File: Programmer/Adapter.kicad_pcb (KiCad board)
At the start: 2 copper layers, 38.1 x 20.3 mm, 5 parts, among them IC1 ARDUINO_PRO_MINI_BASIC, P1 CONN_01X06, P2 CONN_01X02, SW1 SWITCH_SPDT, SW2 SWITCH_SPDT

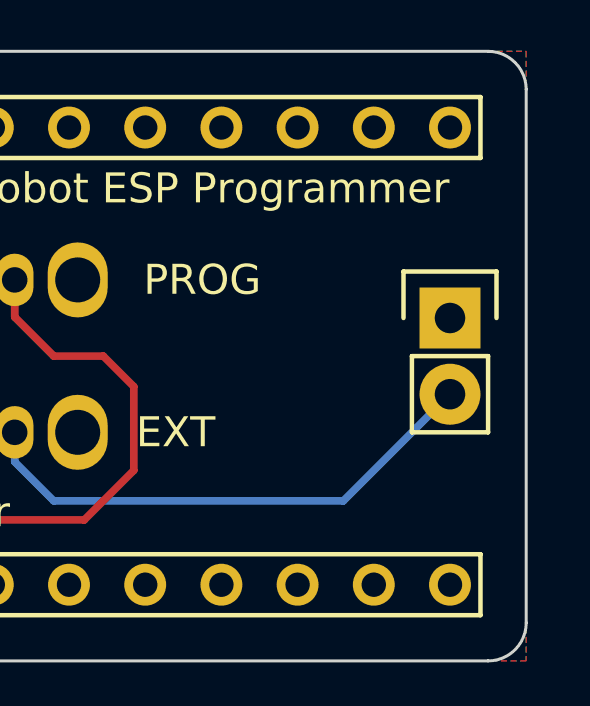
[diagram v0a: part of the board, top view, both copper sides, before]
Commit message: Final production release for v2
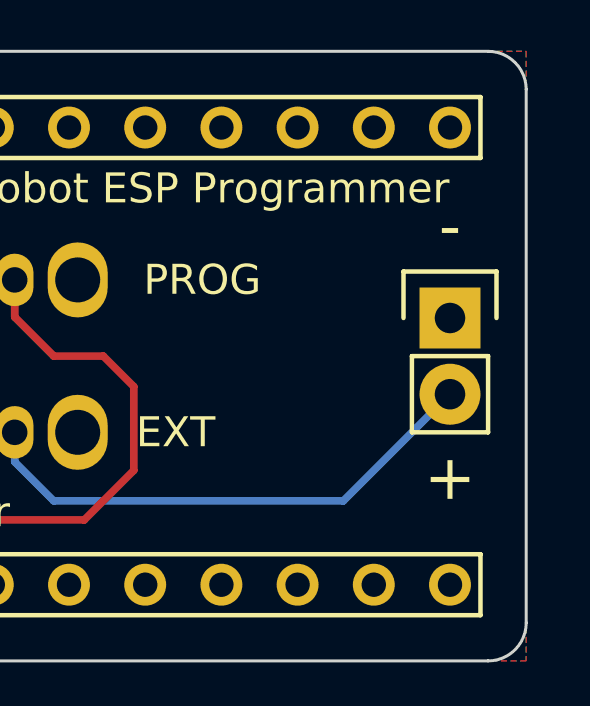
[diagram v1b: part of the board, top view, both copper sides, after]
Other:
- board text added: "+"
- board text added: "-"
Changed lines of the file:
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@@
     (links 10)
     (no_connects 0)
-    (area 128.219999 93.929999 166.420001 114.350001)
+    (area 125.647667 91.511 168.992334 114.350001)
     (thickness 1.6)
-    (drawings 20)
+    (drawings 24)
     (tracks 28)
     (zones 0)
@@
     (pad 5 thru_hole oval (at -4.1 0) (size 2 2.5) (drill 1.5) (layers *.Cu *.Mask F.SilkS))
   )
+  (dimension 20.32 (width 0.3) (layer Eco1.User)
+    (gr_text "20.320 mm" (at 170.768 104.14 270) (layer Eco1.User)
+      (effects (font (size 1.5 1.5) (thickness 0.3)))
+    )
+    (feature1 (pts (xy 167.132 114.3) (xy 172.118 114.3)))
+    (feature2 (pts (xy 167.132 93.98) (xy 172.118 93.98)))
+    (crossbar (pts (xy 169.418 93.98) (xy 169.418 114.3)))
+    (arrow1a (pts (xy 169.418 114.3) (xy 168.831579 113.173496)))
+    (arrow1b (pts (xy 169.418 114.3) (xy 170.004421 113.173496)))
+    (arrow2a (pts (xy 169.418 93.98) (xy 168.831579 95.106504)))
+    (arrow2b (pts (xy 169.418 93.98) (xy 170.004421 95.106504)))
+  )
+  (dimension 38.1 (width 0.3) (layer Eco1.User)
+    (gr_text "38.100 mm" (at 147.32 90.598) (layer Eco1.User)
+      (effects (font (size 1.5 1.5) (thickness 0.3)))
+    )
+    (feature1 (pts (xy 128.27 93.218) (xy 128.27 89.248)))
+    (feature2 (pts (xy 166.37 93.218) (xy 166.37 89.248)))
+    (crossbar (pts (xy 166.37 91.948) (xy 128.27 91.948)))
+    (arrow1a (pts (xy 128.27 91.948) (xy 129.396504 91.361579)))
+    (arrow1b (pts (xy 128.27 91.948) (xy 129.396504 92.534421)))
+    (arrow2a (pts (xy 166.37 91.948) (xy 165.243496 91.361579)))
+    (arrow2b (pts (xy 166.37 91.948) (xy 165.243496 92.534421)))
+  )
+  (gr_text - (at 163.83 99.822) (layer F.SilkS)
+    (effects (font (size 1.5 1.5) (thickness 0.375)) (justify mirror))
+  )
+  (gr_text + (at 163.83 108.204) (layer F.SilkS)
+    (effects (font (size 1.5 1.5) (thickness 0.375)) (justify mirror))
+  )
   (gr_text Power (at 147.066 109.347) (layer F.SilkS)
     (effects (font (size 1 1) (thickness 0.15)))
@@
   (gr_line (start 165.1 93.98) (end 129.54 93.98) (angle 90) (layer Edge.Cuts) (width 0.1))
   (gr_line (start 166.37 113.03) (end 166.37 95.25) (angle 90) (layer Edge.Cuts) (width 0.1))
+  (segment (start 132.08 105.41) (end 135.89 109.22) (width 0.254) (layer F.Cu) (net 1))
+  (segment (start 135.89 109.22) (end 135.89 111.76) (width 0.254) (layer F.Cu) (net 1) (status 20))
   (segment (start 130.81 105.41) (end 132.08 105.41) (width 0.254) (layer F.Cu) (net 1) (status 10))
-  (segment (start 135.89 109.22) (end 135.89 111.76) (width 0.254) (layer F.Cu) (net 1) (status 20))
-  (segment (start 132.08 105.41) (end 135.89 109.22) (width 0.254) (layer F.Cu) (net 1))
+  (segment (start 134.62 107.95) (end 138.43 111.76) (width 0.254) (layer B.Cu) (net 2) (status 20))
   (segment (start 130.81 107.95) (end 134.62 107.95) (width 0.254) (layer B.Cu) (net 2) (status 10))
-  (segment (start 134.62 107.95) (end 138.43 111.76) (width 0.254) (layer B.Cu) (net 2) (status 20))
+  (segment (start 147.32 105.664) (end 145.796 104.14) (width 0.254) (layer B.Cu) (net 3))
+  (segment (start 145.796 104.14) (end 142.24 104.14) (width 0.254) (layer B.Cu) (net 3))
+  (segment (start 142.24 104.14) (end 140.97 102.87) (width 0.254) (layer B.Cu) (net 3))
+  (segment (start 140.97 102.87) (end 140.97 99.06) (width 0.254) (layer B.Cu) (net 3))
+  (segment (start 140.97 99.06) (end 143.51 96.52) (width 0.254) (layer B.Cu) (net 3))
   (segment (start 147.32 106.68) (end 147.32 105.664) (width 0.254) (layer B.Cu) (net 3))
-  (segment (start 140.97 99.06) (end 143.51 96.52) (width 0.254) (layer B.Cu) (net 3))
-  (segment (start 140.97 102.87) (end 140.97 99.06) (width 0.254) (layer B.Cu) (net 3))
-  (segment (start 142.24 104.14) (end 140.97 102.87) (width 0.254) (layer B.Cu) (net 3))
-  (segment (start 145.796 104.14) (end 142.24 104.14) (width 0.254) (layer B.Cu) (net 3))
-  (segment (start 147.32 105.664) (end 145.796 104.14) (width 0.254) (layer B.Cu) (net 3))
+  (segment (start 135.128 102.87) (end 141.478 109.22) (width 0.254) (layer B.Cu) (net 5))
+  (segment (start 141.478 109.22) (end 144.272 109.22) (width 0.254) (layer B.Cu) (net 5))
+  (segment (start 144.272 109.22) (end 145.32 108.172) (width 0.254) (layer B.Cu) (net 5))
+  (segment (start 145.32 108.172) (end 145.32 106.68) (width 0.254) (layer B.Cu) (net 5))
   (segment (start 130.81 102.87) (end 135.128 102.87) (width 0.254) (layer B.Cu) (net 5))
-  (segment (start 145.32 108.172) (end 145.32 106.68) (width 0.254) (layer B.Cu) (net 5))
-  (segment (start 144.272 109.22) (end 145.32 108.172) (width 0.254) (layer B.Cu) (net 5))
-  (segment (start 141.478 109.22) (end 144.272 109.22) (width 0.254) (layer B.Cu) (net 5))
-  (segment (start 135.128 102.87) (end 141.478 109.22) (width 0.254) (layer B.Cu) (net 5))
+  (segment (start 149.32 107.664) (end 150.622 108.966) (width 0.254) (layer B.Cu) (net 6))
+  (segment (start 150.622 108.966) (end 160.274 108.966) (width 0.254) (layer B.Cu) (net 6))
+  (segment (start 160.274 108.966) (end 163.83 105.41) (width 0.254) (layer B.Cu) (net 6))
   (segment (start 149.32 106.68) (end 149.32 107.664) (width 0.254) (layer B.Cu) (net 6))
-  (segment (start 160.274 108.966) (end 163.83 105.41) (width 0.254) (layer B.Cu) (net 6))
-  (segment (start 150.622 108.966) (end 160.274 108.966) (width 0.254) (layer B.Cu) (net 6))
-  (segment (start 149.32 107.664) (end 150.622 108.966) (width 0.254) (layer B.Cu) (net 6))
+  (segment (start 149.32 102.838) (end 150.622 104.14) (width 0.254) (layer F.Cu) (net 7))
+  (segment (start 150.622 104.14) (end 152.273 104.14) (width 0.254) (layer F.Cu) (net 7))
+  (segment (start 152.273 104.14) (end 153.289 105.156) (width 0.254) (layer F.Cu) (net 7))
+  (segment (start 153.289 105.156) (end 153.289 107.95) (width 0.254) (layer F.Cu) (net 7))
+  (segment (start 153.289 107.95) (end 151.638 109.601) (width 0.254) (layer F.Cu) (net 7))
+  (segment (start 151.638 109.601) (end 148.209 109.601) (width 0.254) (layer F.Cu) (net 7))
+  (segment (start 148.209 109.601) (end 146.05 111.76) (width 0.254) (layer F.Cu) (net 7))
   (segment (start 149.32 101.6) (end 149.32 102.838) (width 0.254) (layer F.Cu) (net 7))
-  (segment (start 148.209 109.601) (end 146.05 111.76) (width 0.254) (layer F.Cu) (net 7))
-  (segment (start 151.638 109.601) (end 148.209 109.601) (width 0.254) (layer F.Cu) (net 7))
-  (segment (start 153.289 107.95) (end 151.638 109.601) (width 0.254) (layer F.Cu) (net 7))
-  (segment (start 153.289 105.156) (end 153.289 107.95) (width 0.254) (layer F.Cu) (net 7))
-  (segment (start 152.273 104.14) (end 153.289 105.156) (width 0.254) (layer F.Cu) (net 7))
-  (segment (start 150.622 104.14) (end 152.273 104.14) (width 0.254) (layer F.Cu) (net 7))
-  (segment (start 149.32 102.838) (end 150.622 104.14) (width 0.254) (layer F.Cu) (net 7))
   (zone (net 4) (net_name GND) (layer F.Cu) (hatch edge 0.508)
     (connect_pads (clearance 0.508))
